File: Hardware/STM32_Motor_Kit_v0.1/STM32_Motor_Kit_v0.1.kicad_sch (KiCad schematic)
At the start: 28 parts

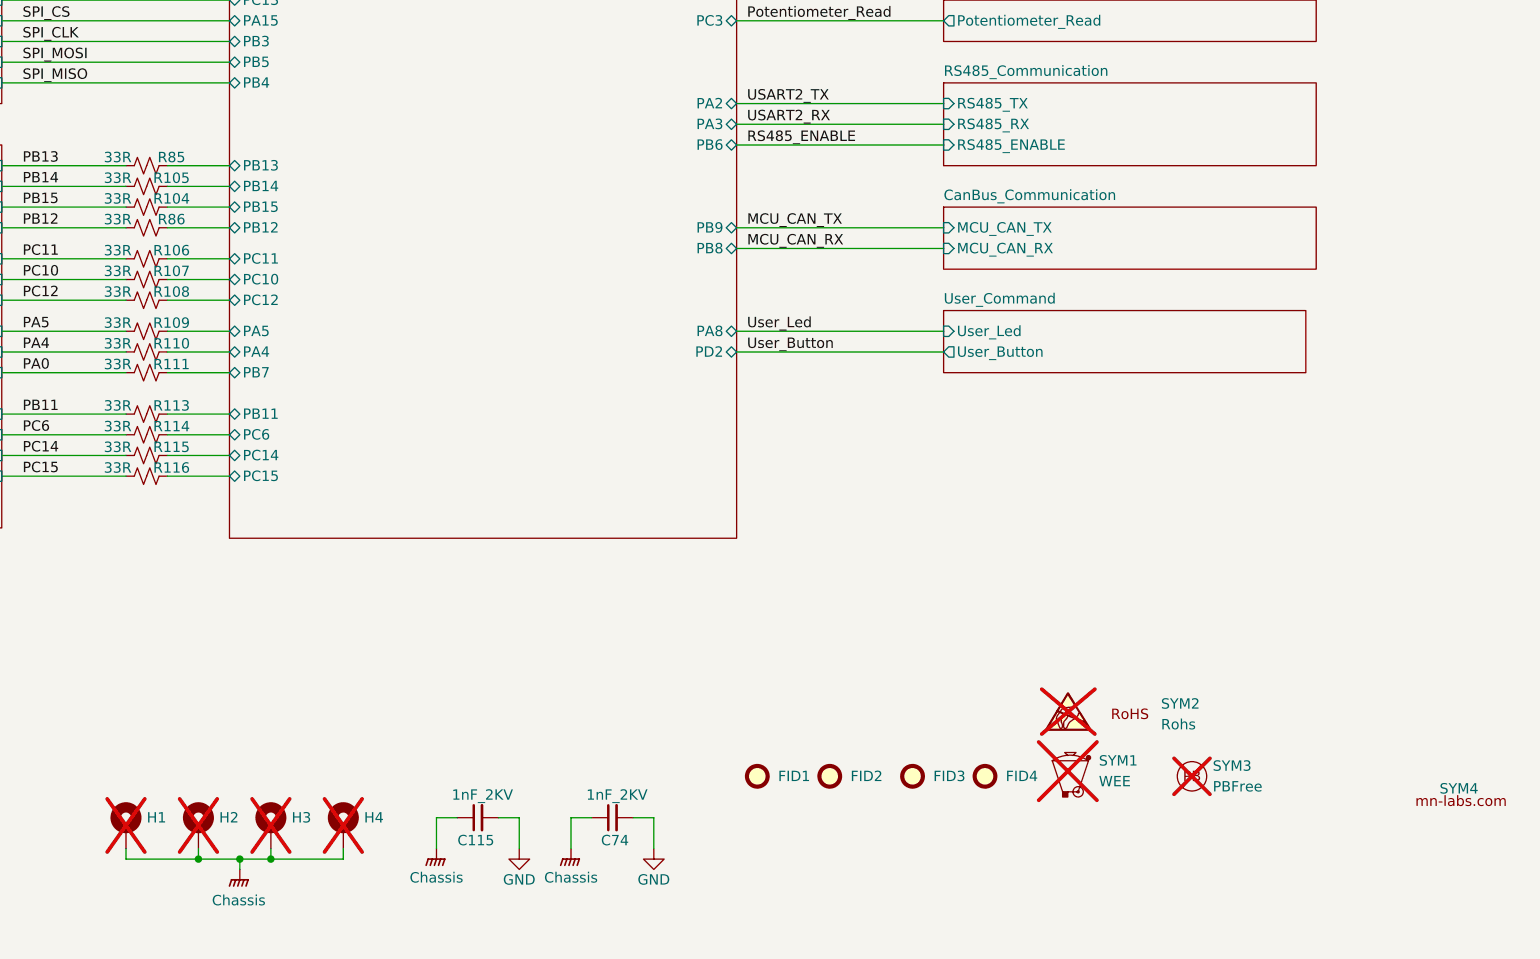
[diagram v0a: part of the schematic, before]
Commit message: 12.01.2025
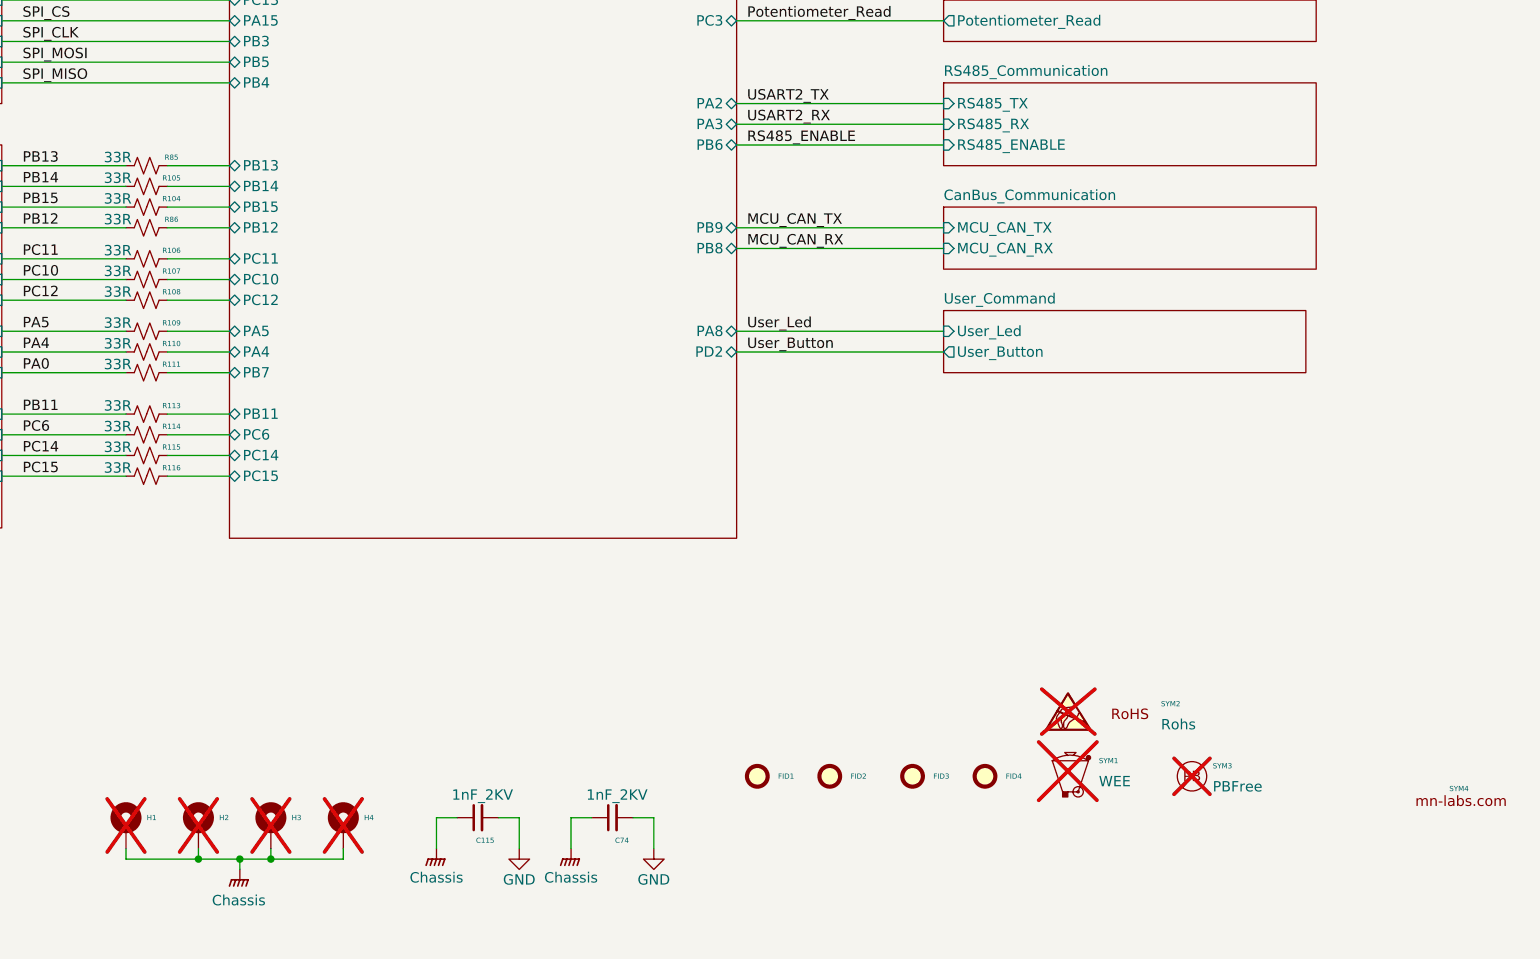
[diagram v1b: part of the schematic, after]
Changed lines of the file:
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@@
 			(effects
 				(font
-					(size 1.27 1.27)
+					(face "Arial")
+					(size 0.635 0.635)
 				)
 				(hide yes)
@@
 			(effects
 				(font
-					(size 1.27 1.27)
+					(face "Arial")
+					(size 0.635 0.635)
 				)
 				(hide yes)
@@
 			(effects
 				(font
-					(size 1.27 1.27)
+					(face "Arial")
+					(size 0.635 0.635)
 				)
 			)
@@
 			(effects
 				(font
-					(size 1.27 1.27)
+					(face "Arial")
+					(size 0.635 0.635)
 				)
 			)
@@
 			(effects
 				(font
-					(size 1.27 1.27)
+					(face "Arial")
+					(size 0.635 0.635)
 				)
 				(justify left)
@@
 			(effects
 				(font
-					(size 1.27 1.27)
+					(face "Arial")
+					(size 0.635 0.635)
 				)
 			)
@@
 			(effects
 				(font
-					(size 1.27 1.27)
+					(face "Arial")
+					(size 0.635 0.635)
 				)
 				(hide yes)
@@
 			(effects
 				(font
-					(size 1.27 1.27)
+					(face "Arial")
+					(size 0.635 0.635)
 				)
 			)
@@
 			(effects
 				(font
-					(size 1.27 1.27)
+					(face "Arial")
+					(size 0.635 0.635)
 				)
 			)
@@
 			(effects
 				(font
-					(size 1.27 1.27)
+					(face "Arial")
+					(size 0.635 0.635)
 				)
 				(justify left)
@@
 			(effects
 				(font
-					(size 1.27 1.27)
+					(face "Arial")
+					(size 0.635 0.635)
 				)
 			)
@@
 			(effects
 				(font
-					(size 1.27 1.27)
+					(face "Arial")
+					(size 0.635 0.635)
 				)
 				(justify left)
@@
 			(effects
 				(font
-					(size 1.27 1.27)
+					(face "Arial")
+					(size 0.635 0.635)
 				)
 				(justify left)
@@
 			(effects
 				(font
-					(size 1.27 1.27)
+					(face "Arial")
+					(size 0.635 0.635)
 				)
 				(justify left)
@@
 			(effects
 				(font
-					(size 1.27 1.27)
+					(face "Arial")
+					(size 0.635 0.635)
 				)
 				(justify left)
@@
 			(effects
 				(font
-					(size 1.27 1.27)
+					(face "Arial")
+					(size 0.635 0.635)
 				)
 				(justify left)
@@
 			(effects
 				(font
-					(size 1.27 1.27)
+					(face "Arial")
+					(size 0.635 0.635)
 				)
 				(justify left)
@@
 			(effects
 				(font
-					(size 1.27 1.27)
+					(face "Arial")
+					(size 0.635 0.635)
 				)
 			)
@@
 			(effects
 				(font
-					(size 1.27 1.27)
+					(face "Arial")
+					(size 0.635 0.635)
 				)
 			)
@@
 			(effects
 				(font
-					(size 1.27 1.27)
+					(face "Arial")
+					(size 0.635 0.635)
 				)
 			)
@@
 			(effects
 				(font
-					(size 1.27 1.27)
+					(face "Arial")
+					(size 0.635 0.635)
 				)
 				(justify left)
@@
 			(effects
 				(font
-					(size 1.27 1.27)
+					(face "Arial")
+					(size 0.635 0.635)
 				)
 				(justify left)
@@
 			(effects
 				(font
-					(size 1.27 1.27)
+					(face "Arial")
+					(size 0.635 0.635)
 				)
 				(justify left)
@@
 			(effects
 				(font
-					(size 1.27 1.27)
+					(face "Arial")
+					(size 0.635 0.635)
 				)
 			)
@@
 			(effects
 				(font
-					(size 1.27 1.27)
+					(face "Arial")
+					(size 0.635 0.635)
 				)
 				(justify left)
@@
 			(effects
 				(font
-					(size 1.27 1.27)
+					(face "Arial")
+					(size 0.635 0.635)
 				)
 			)
@@
 			(effects
 				(font
-					(size 1.27 1.27)
+					(face "Arial")
+					(size 0.635 0.635)
 				)
 				(hide yes)
@@
 			(effects
 				(font
-					(size 1.27 1.27)
+					(face "Arial")
+					(size 0.635 0.635)
 				)
 			)
@@
 			(effects
 				(font
-					(size 1.27 1.27)
+					(face "Arial")
+					(size 0.635 0.635)
 				)
 				(hide yes)
@@
 			(effects
 				(font
-					(size 1.27 1.27)
+					(face "Arial")
+					(size 0.635 0.635)
 				)
 				(justify left)
@@
 			(effects
 				(font
-					(size 1.27 1.27)
+					(face "Arial")
+					(size 0.635 0.635)
 				)
 			)
@@
 			(effects
 				(font
-					(size 1.27 1.27)
+					(face "Arial")
+					(size 0.635 0.635)
 				)
 			)
@@
 			(effects
 				(font
-					(size 1.27 1.27)
+					(face "Arial")
+					(size 0.635 0.635)
 				)
 				(hide yes)
@@
 			(effects
 				(font
-					(size 1.27 1.27)
-				)
-			)
+					(face "Arial")
+					(size 0.635 0.635)
+				)
+			)

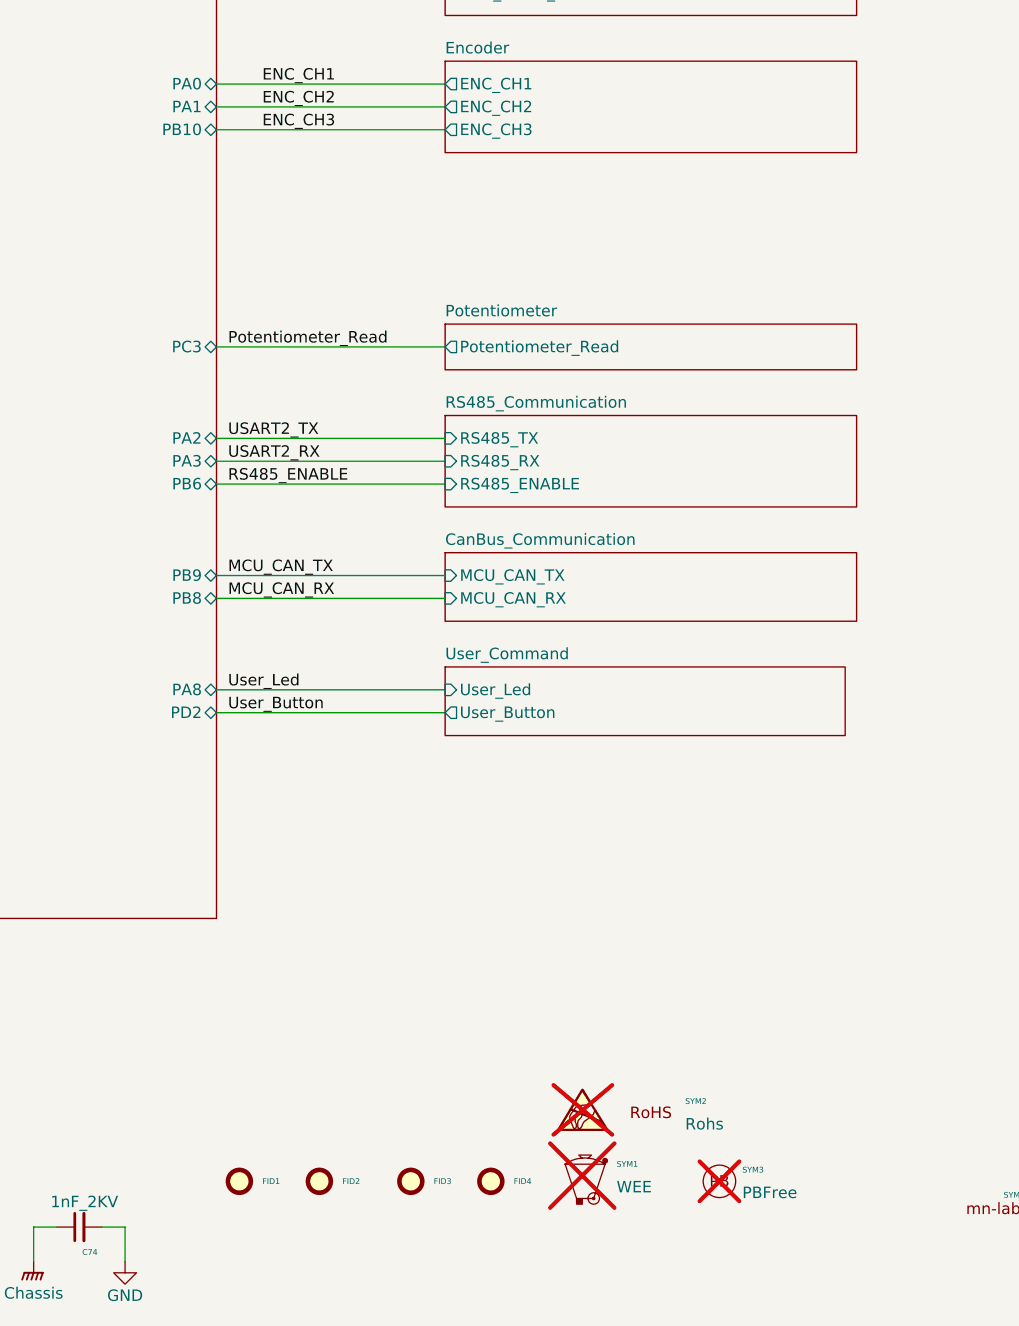
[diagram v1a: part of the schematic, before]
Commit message: Şema üzerinde değişiklikler devam ediyor
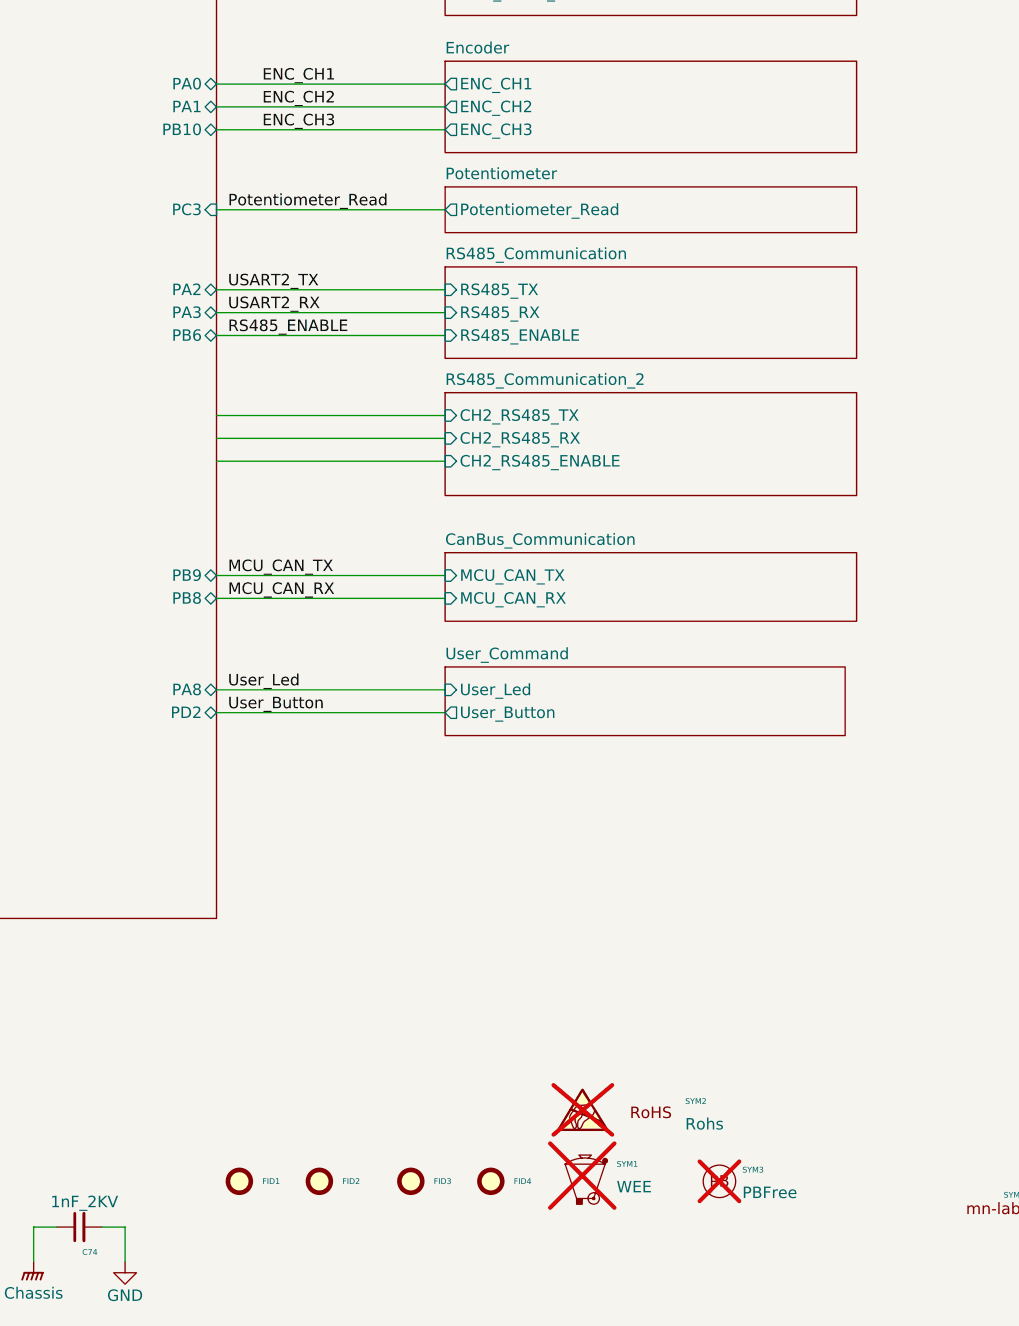
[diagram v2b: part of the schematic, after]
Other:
- added sheet RS485_Communication_2 (RS485_Communication_2.kicad_sch)
